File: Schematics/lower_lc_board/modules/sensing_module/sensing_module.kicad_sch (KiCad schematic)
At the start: 23 parts, among them J4 HALL-1, J5 HALL-2, Q3 2N7002, U11 SI2301CDS-T1-GE3, U9 ADC_ADS131M04IPWR

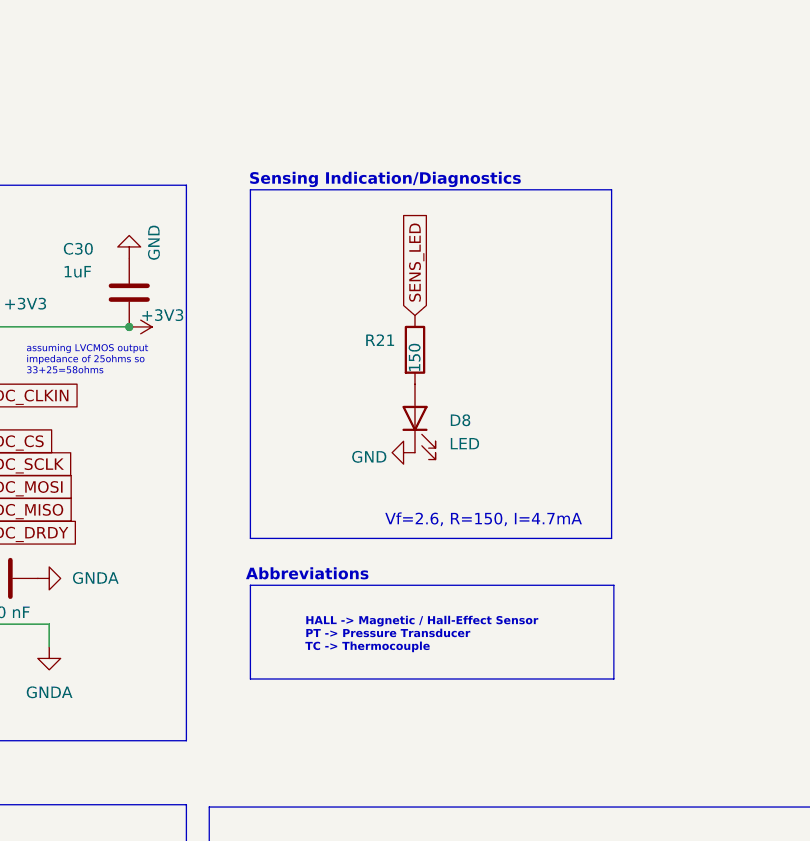
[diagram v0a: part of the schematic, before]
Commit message: more layout work, add testing code
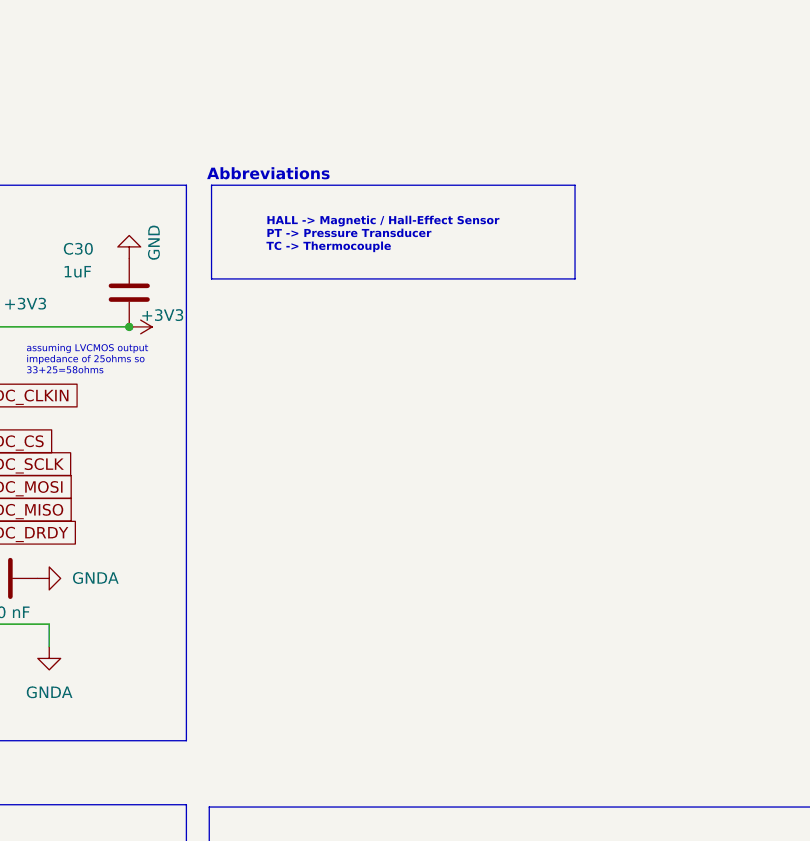
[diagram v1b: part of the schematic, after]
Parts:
- removed D8: LED, LED_SMD:LED_0603_1608Metric, symbol Device:LED
- removed R21: 150, Resistor_SMD:R_0603_1608Metric, symbol Device:R
- R23: footprint Resistor_SMD:R_0603_1608Metric -> Resistor_SMD:R_0402_1005Metric
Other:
- note removed: "Sensing Indication/Diagnostics"
- note removed: "Vf=2.6, R=150, I=4.7mA"
